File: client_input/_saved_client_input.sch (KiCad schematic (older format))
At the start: 29 parts, among them P1 Analog In, P2 FTDI, P3 Ribbon, P4 spare I/O, P5 Ribbon, P6 Ribbon, P7 Ribbon, P8 Ribbon, SW1 PAIR_MODE, SW2 RESET, SW3 Bootload, SW4 DIPS_08, U1 MCP3208, U2 ESP-12_Breakout, U3 MCP23017

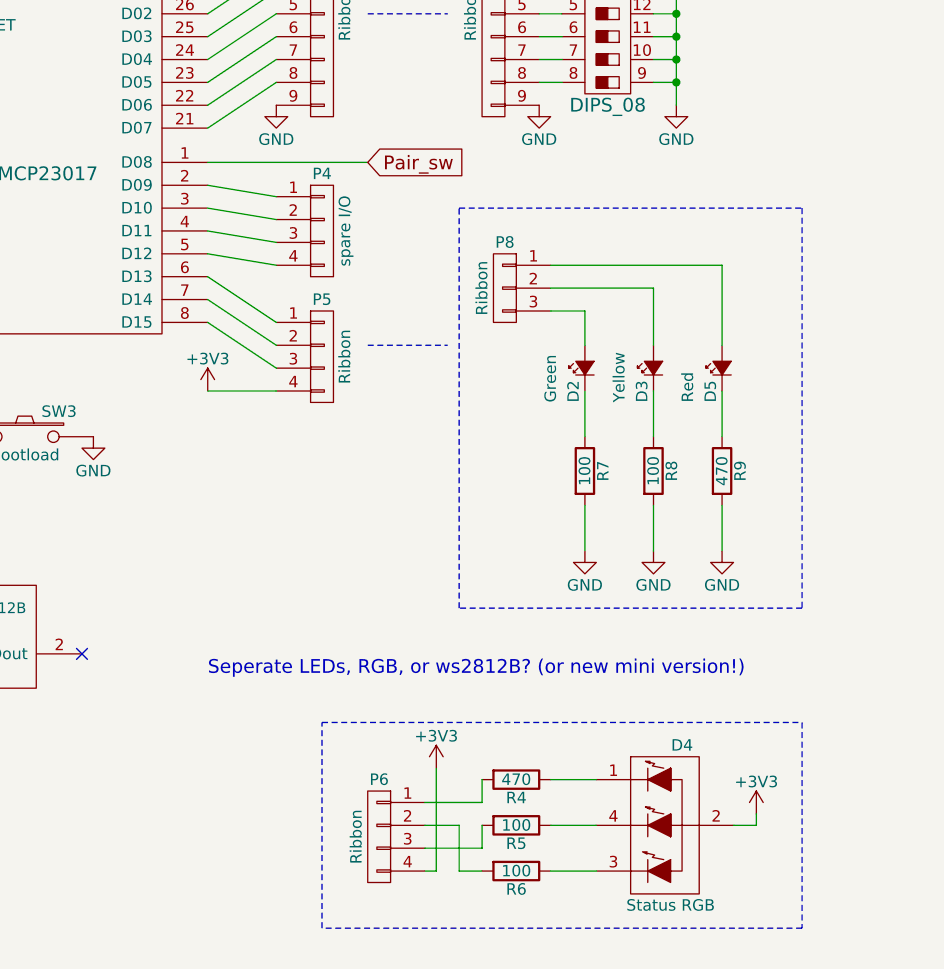
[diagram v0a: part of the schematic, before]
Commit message: PCD laid out.
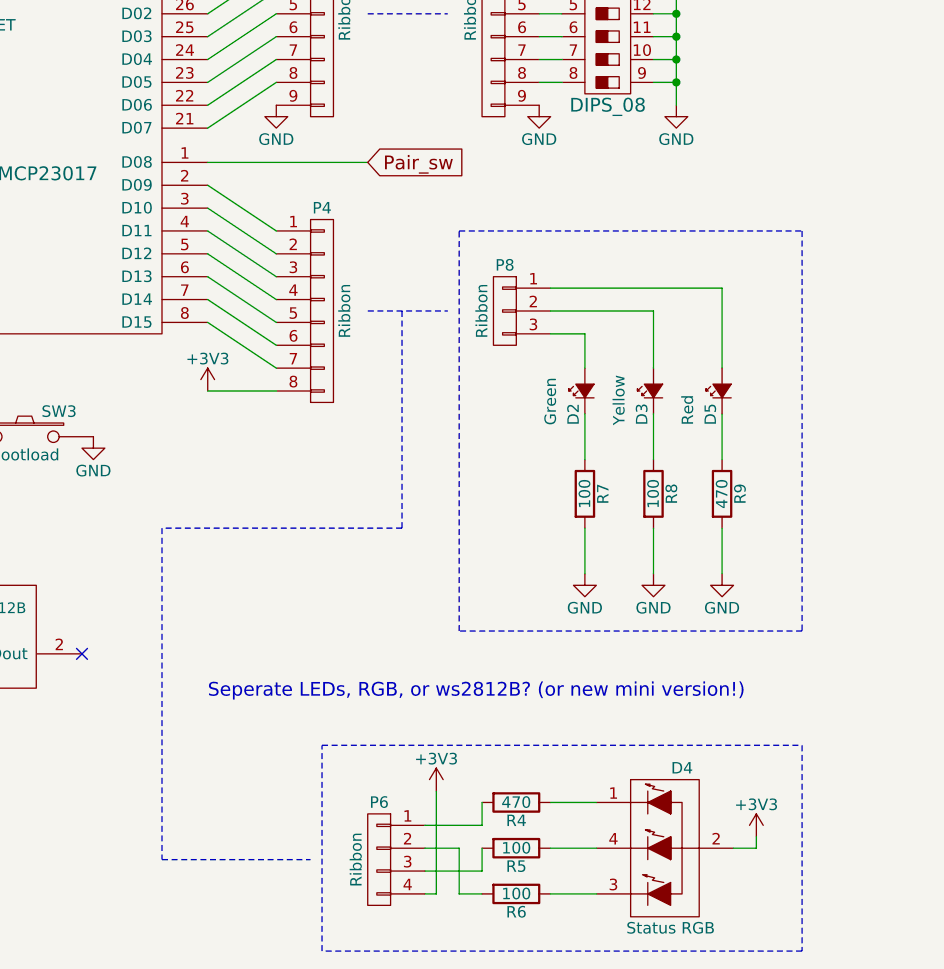
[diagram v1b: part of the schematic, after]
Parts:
- removed P4: spare I/O, Socket_Strips:Socket_Strip_Straight_1x04, symbol CONN_01X04
- removed P5: Ribbon, symbol CONN_01X04
- added P4: Ribbon, Socket_Strips:Socket_Strip_Straight_1x08, symbol CONN_01X08
- P6: footprint (none) -> Socket_Strips:Socket_Strip_Straight_1x04
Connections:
- net +3V3: now also P4.8 (P8)
- net at U3.2 (D09): now also P4.1 (P1)
- net at U3.3 (D10): now also P4.2 (P2)
- net at U3.4 (D11): now also P4.3 (P3)
- net at U3.5 (D12): now also P4.4 (P4)
- net at U3.6 (D13): now also P4.5 (P5)
- net at U3.7 (D14): now also P4.6 (P6)
- net at U3.8 (D15): now also P4.7 (P7)
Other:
- moved on the sheet: D2, D3, D4, D5, P6, P8, R4, R5, R6, R7, R8, R9
